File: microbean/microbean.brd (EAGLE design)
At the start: 33 x 27.6 mm, 20 parts, among them IC1 L78L33/L78L05, IC2 ST485/ST3485, IC3 PIC16F1827SO18

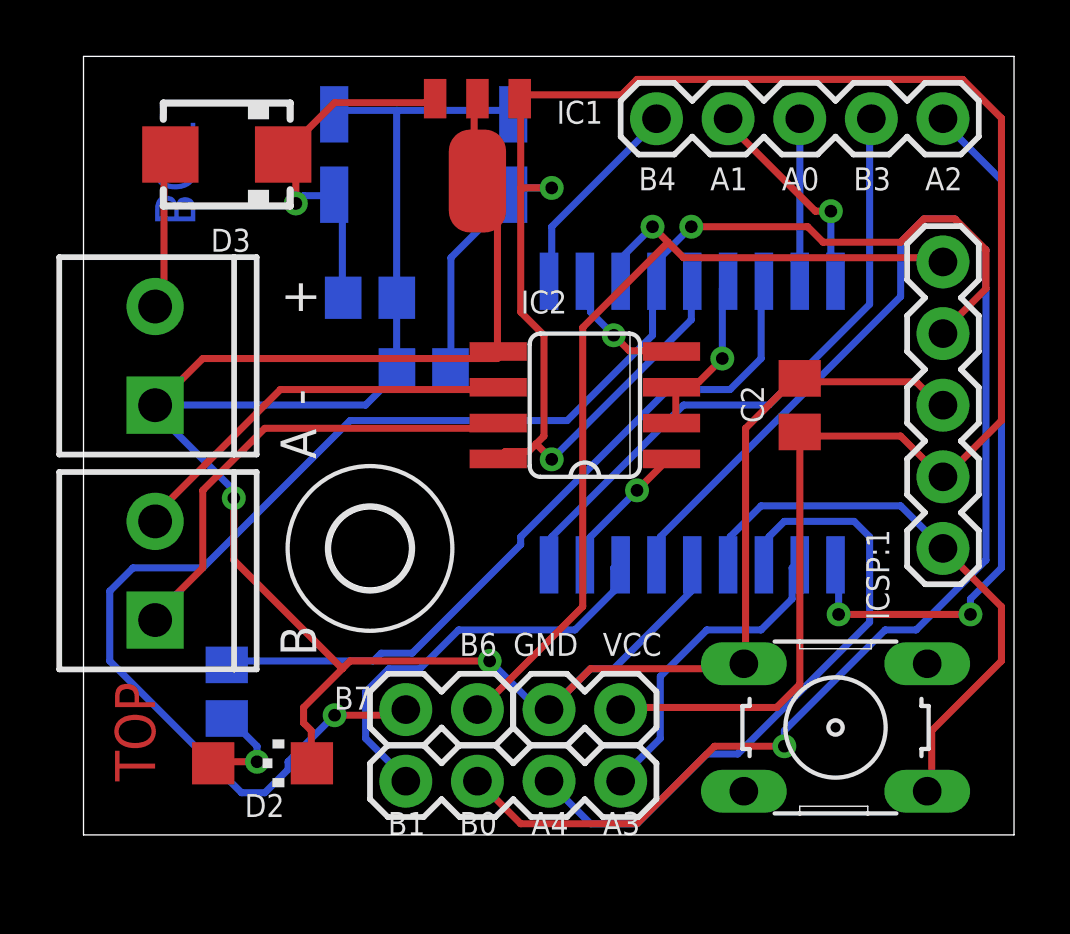
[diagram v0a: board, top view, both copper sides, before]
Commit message: - Ready for printing, optimized
git-svn-id: svn://mule/net/hardware/trunk@565 1a6b750e-079f-425f-90e7-3a118970be6b
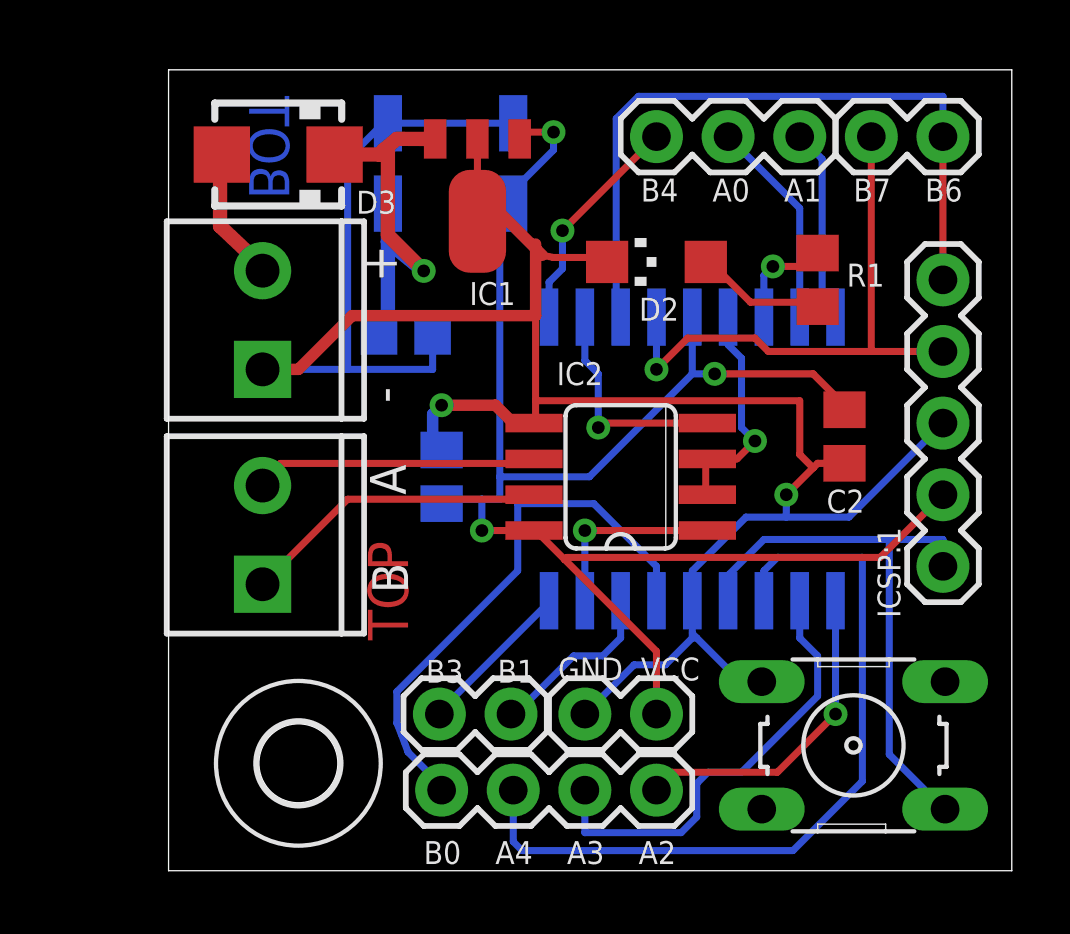
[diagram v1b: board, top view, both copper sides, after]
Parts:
- added J7: (no value), custom:1X02
- J3: device custom:1X05 -> custom:1X03
- moved J6 26.2 mm to (29.2, 36.2)
- moved R1 25.5 mm to (27.3, 31.1), flipped to the top
- moved D2 22.6 mm to (21.6, 31.8), turned to 90 degrees
- moved U$4 8.03 mm to (8.89, 14.0)
- moved J1 4.02 mm to (7.62, 27.9)
- moved J2 4.02 mm to (7.62, 20.3)
- moved C5 3.86 mm to (14.0, 24.1), turned to 90 degrees
- moved IC2 2.84 mm to (20.3, 24.1)
- moved C2 1.94 mm to (28.3, 25.6), turned to 270 degrees
- moved C3 1.93 mm to (12.1, 35.2)
- moved D3 1.83 mm to (8.18, 35.6)
- moved C1 1.80 mm to (12.7, 29.2)
- moved IC1 1.43 mm to (15.2, 34.1)
- moved J4 1.31 mm to (21.6, 13.0)
- moved J5 1.28 mm to (21.6, 15.7)
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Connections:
- net N$23 renamed RA6
- net N$9 renamed RA7
- net RA0: now also J3.2; no longer J3.3
- net RA1: now also J3.3; no longer J3.2
- net RA2: now also J4.1; no longer J3.5
- net RA3: now also J4.2; no longer J4.1
- net RA4: now also J4.3; no longer J4.2
- net RB0: now also J4.4; no longer J4.3
- net RB1: now also J7.2; no longer J4.4
- net RB3: now also J7.1; no longer J3.4
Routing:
- net RB7: track 58.9 -> 20.3 mm, vias 2 -> 1
- net RB0: track 52.7 -> 19.6 mm, vias 1 -> 0
- net VCC: track 86.0 -> 60.0 mm, vias 2 -> 3
- net RA7: track 26.3 -> 3.80 mm, vias 0 -> 1
- net RB3: track 22.3 -> 5.62 mm
- net GND: track 103.7 -> 89.7 mm
- net RA2: track 25.4 -> 11.5 mm, vias 2 -> 1
- net RB1: track 15.1 -> 6.33 mm
- net RB6: track 32.6 -> 25.5 mm, vias 1 -> 0
- net B: track 16.8 -> 10.9 mm
- net RA4: track 23.1 -> 28.1 mm
- net RA3: track 11.5 -> 16.1 mm
- net A: track 14.6 -> 10.1 mm
- net RB5: track 4.60 -> 8.05 mm
- net N$2: track 13.4 -> 15.2 mm
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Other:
- board size 33 x 27.6 mm -> 29.9 x 28.4 mm
